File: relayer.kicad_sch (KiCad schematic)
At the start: 4 parts, among them U16 HN2199

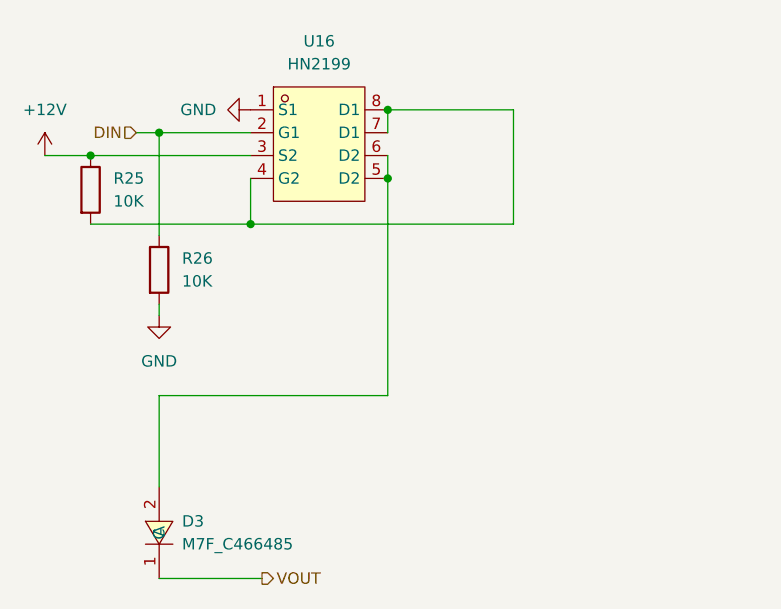
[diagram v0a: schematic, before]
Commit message: almost ready for prod
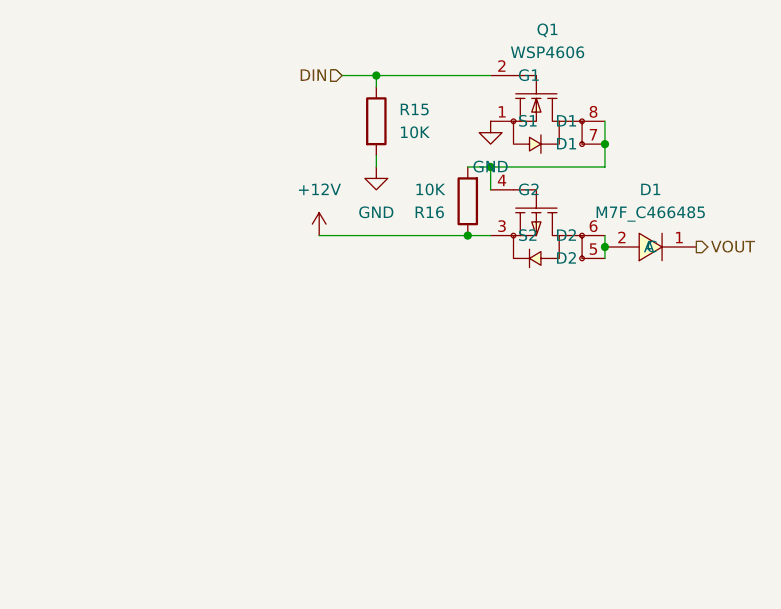
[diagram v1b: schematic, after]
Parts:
- removed D3: M7F_C466485, m7f:SMAF_L3.5-W2.6-LS4.7-RD, symbol m7f:M7F_C466485
- removed R25, R26: 10K, Resistor_SMD:R_0603_1608Metric, symbol Device:R
- removed U16: HN2199, hn2199:DFN-8_L5.8-W4.9-P1.27-LS6.0-BL, symbol hn2199:HN2199
- added D1: M7F_C466485, m7f:SMAF_L3.5-W2.6-LS4.7-RD, symbol m7f:M7F_C466485
- added Q1: WSP4606, blastLib:SOP-8_L4.9-W3.9-P1.27-LS6.0-BL, symbol blastLib:WSP4606
- added R15, R16: 10K, Resistor_SMD:R_0603_1608Metric, symbol Device:R
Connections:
- net +12V: now also Q1.3 (S2), R16.1
- net DIN: now also Q1.2 (G1), R15.1
- net GND: now also Q1.1 (S1), R15.2
- net VOUT: now also D1.1 (C)
- new net: D1.2 (A), Q1.5 (D2), Q1.6 (D2)
- new net: Q1.4 (G2), Q1.7 (D1), Q1.8 (D1), R16.2
